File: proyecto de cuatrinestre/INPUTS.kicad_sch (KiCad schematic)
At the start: 28 parts, among them U2 FODM2705, U3 FODM2705, U4 FODM2705, U5 FODM2705

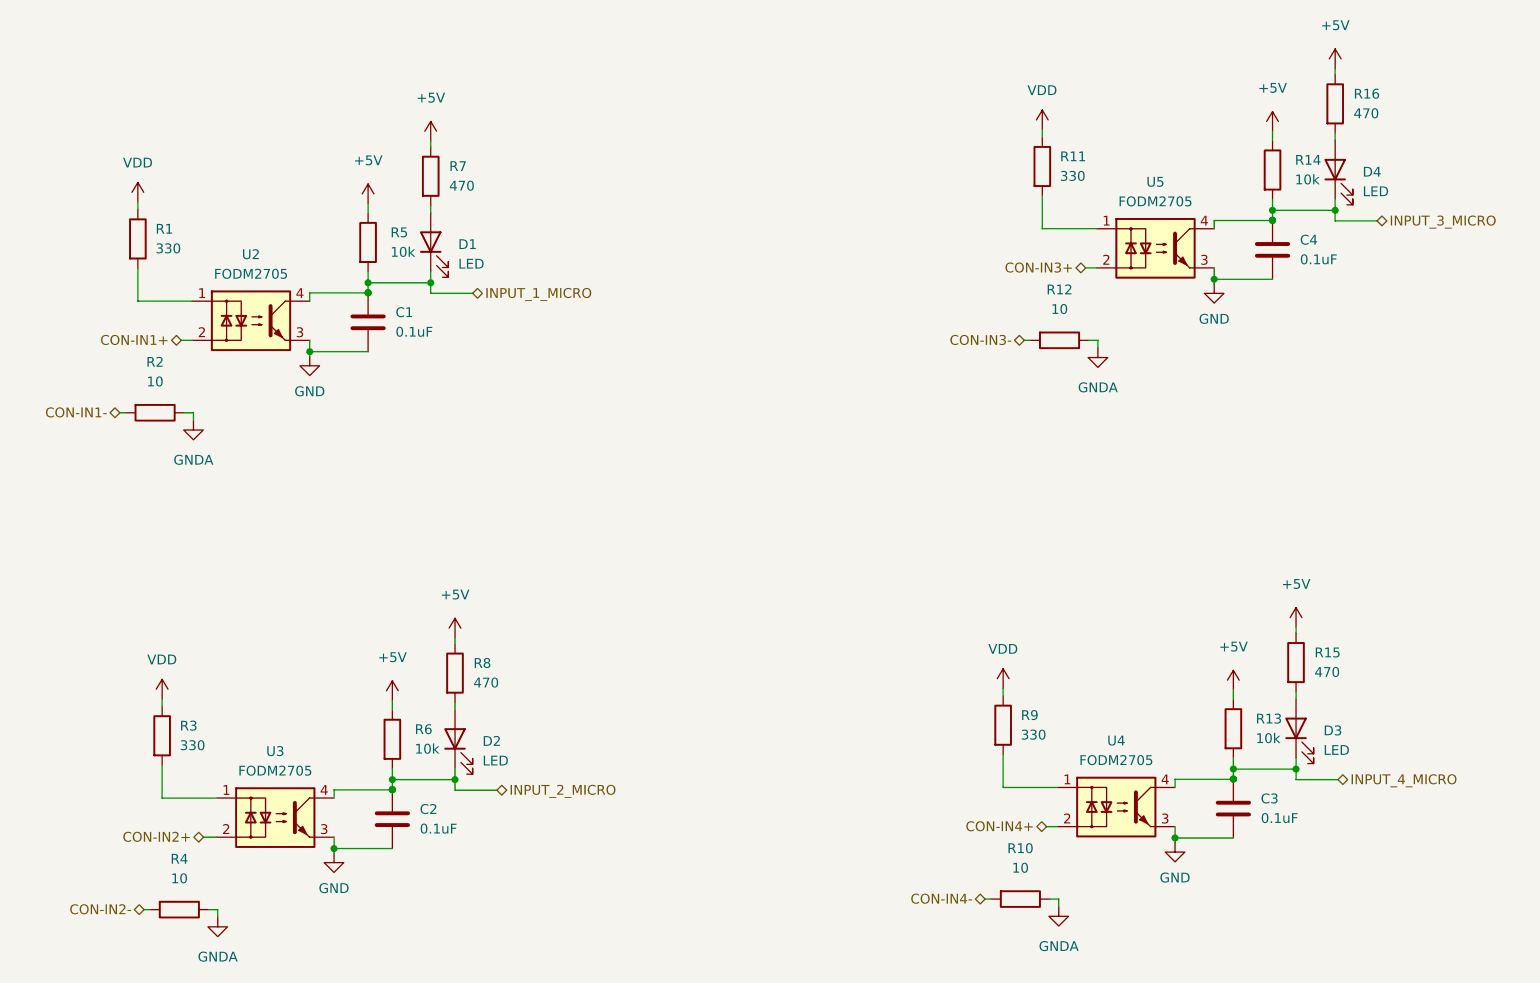
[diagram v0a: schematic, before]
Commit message: absolutamente todo
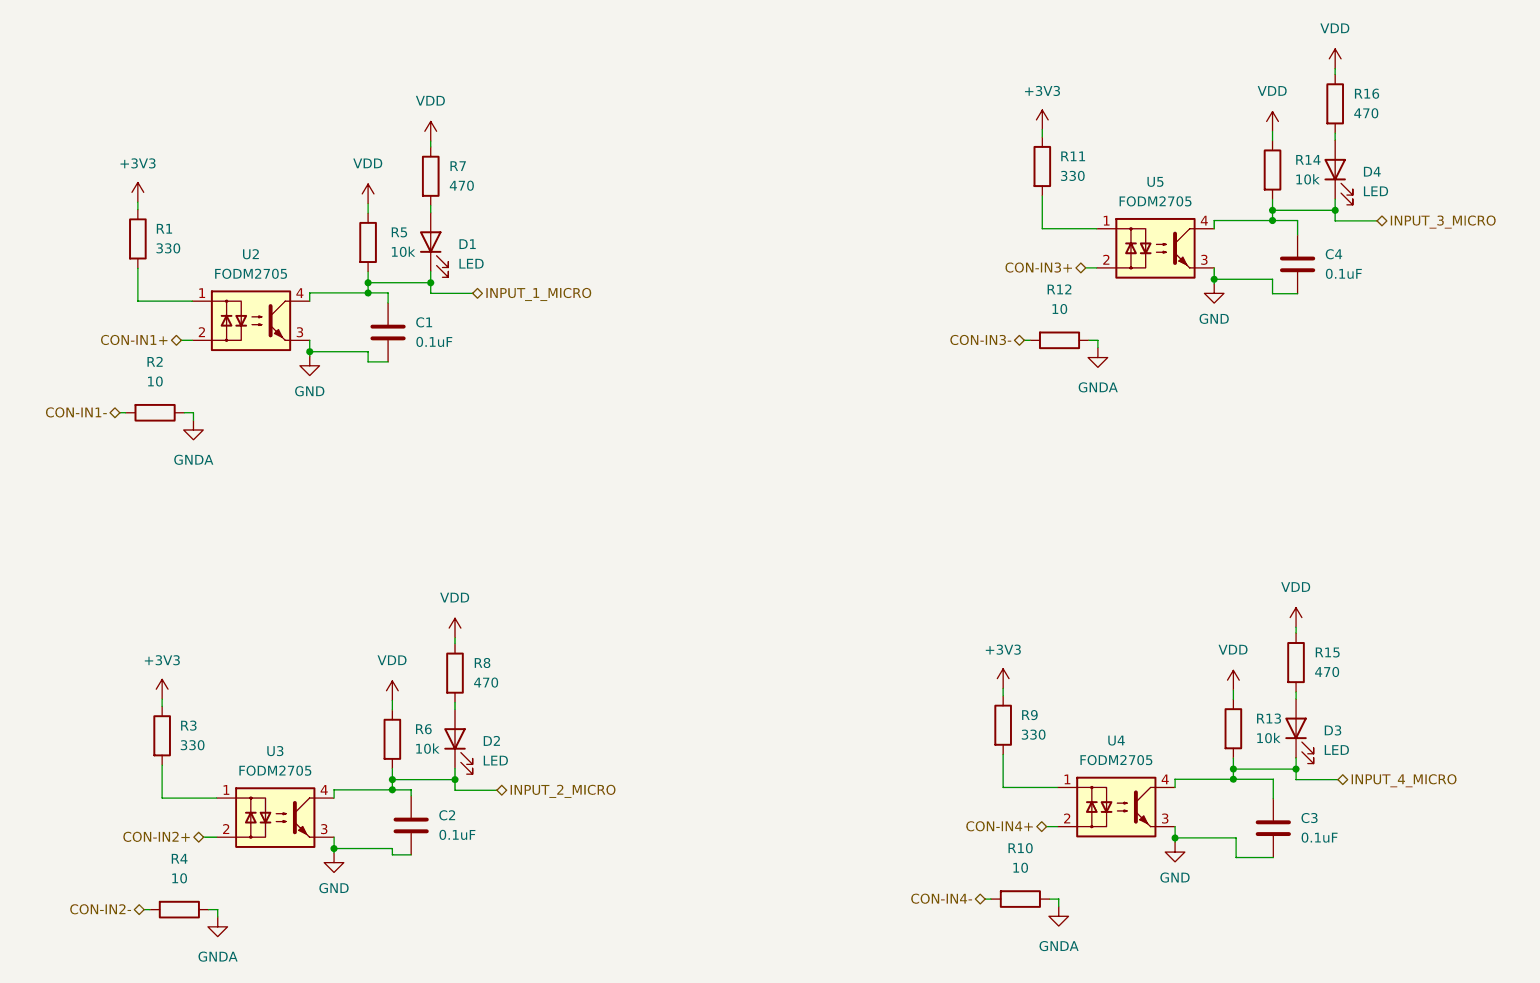
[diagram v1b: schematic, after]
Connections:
- net +5V is gone; now on net VDD: R13.1, R14.1, R15.1, R16.1, R5.1, R6.1, R7.1, R8.1
- net INPUT_1_MICRO: now also C1.1, U2.4
- net INPUT_2_MICRO: now also C2.1, U3.4
- net INPUT_3_MICRO: now also C4.1, U5.4
- net INPUT_4_MICRO: now also C3.1, U4.4
- net VDD: no longer R1.1, R11.1, R3.1, R9.1
- new net +3V3: R1.1, R11.1, R3.1, R9.1
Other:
- moved on the sheet: C1, C2, C3, C4
